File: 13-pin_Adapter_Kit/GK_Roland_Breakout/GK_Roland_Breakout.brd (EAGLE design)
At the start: 40 x 29.6 mm, 39 parts, among them T2 2N4401, U1 RC4558, U2 MIC5205-5V

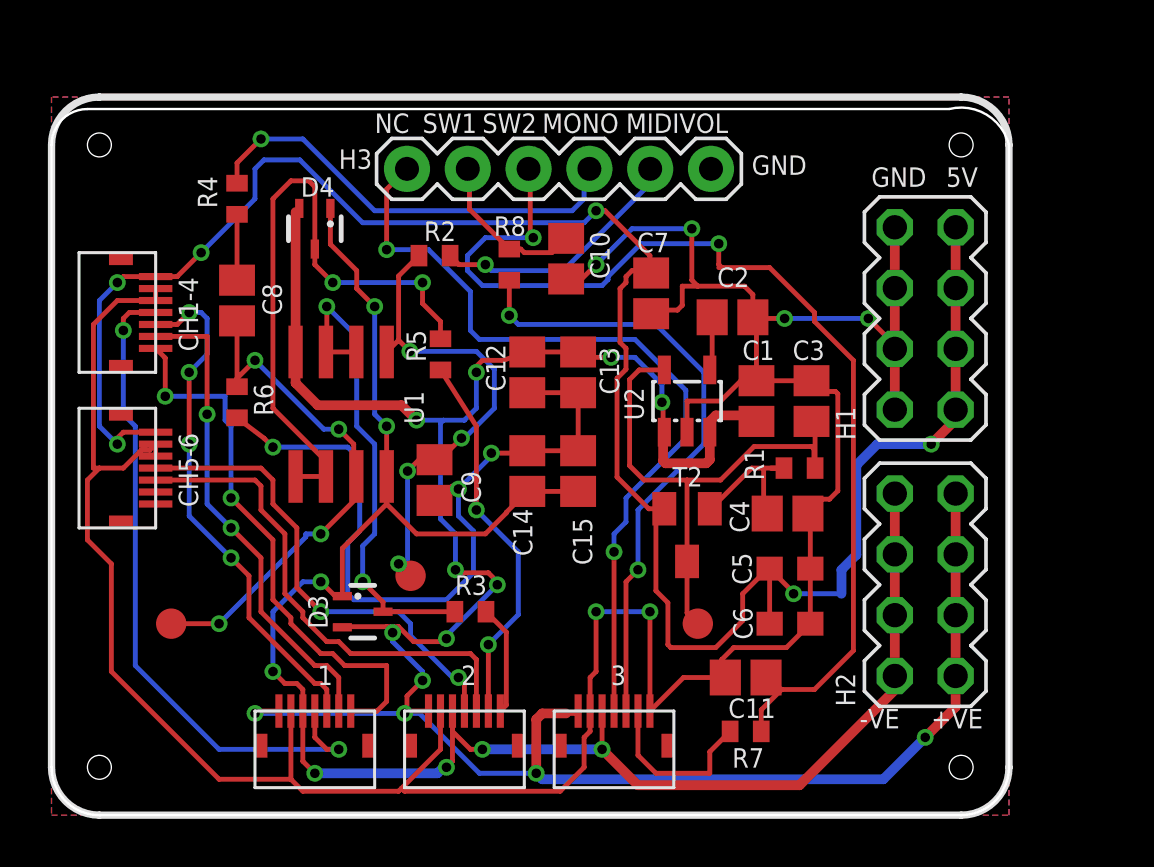
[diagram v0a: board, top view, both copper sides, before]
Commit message: Updated BOM
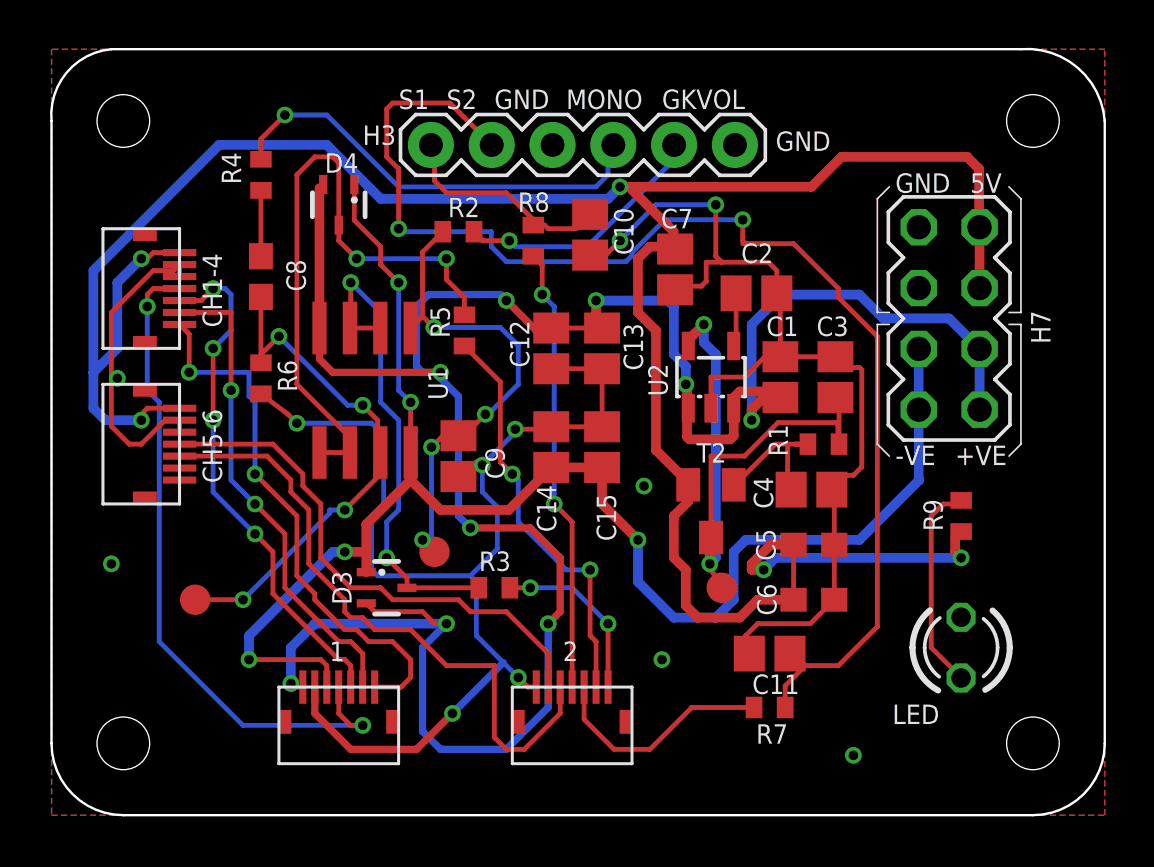
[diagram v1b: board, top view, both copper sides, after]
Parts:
- removed H6, H8: 7P_ZIF_59453-071110EDHLF, CYCFI_Con:7P_ZIF_59453-071110EDHLF
- added LED: (no value), led:LED3MM
- added R9: 4.7k, resistor:R0402
- C10, C11, C9: value 0.01u -> 0.01uF
- C12, C14: value 4.7u -> 4.7uF
- C13, C15: value 0.1u -> 0.1uF
- C5: value 1nf -> 1nF
- C6: value 1uf -> 1uF
- C8: value 0.47u -> 0.47uF; device resistor:C0805 -> resistor:C0603
- H1, H2: value (none) -> 7P_ZIF_59453-071110EDHLF; device con-lstb:MA04-2 -> CYCFI_Con:7P_ZIF_59453-071110EDHLF
- H3: value 6P-2.54-TH -> (none)
- H7: value 7P_ZIF_59453-071110EDHLF -> (none); device CYCFI_Con:7P_ZIF_59453-071110EDHLF -> con-lstb:MA04-2
- R3, R5: value 100 -> 100R
- moved H2 33.3 mm to (3.75, 15.5), turned to 270 degrees
- moved H1 32.8 mm to (3.75, 22.0), turned to 270 degrees
- moved H7 27.1 mm to (37.5, 20.8), turned to 90 degrees
- moved H5 21.8 mm to (21.8, 3.75), turned to 0 degrees
- moved H4 19.6 mm to (12.0, 3.75), turned to 0 degrees
- moved TP1 1.80 mm to (28.0, 9.50)
- moved C1 1.41 mm to (30.4, 18.3)
- moved C10 1.41 mm to (22.5, 24.2)
- moved C11 1.41 mm to (30.0, 6.75)
- moved C12 1.41 mm to (20.9, 19.5)
- moved C13 1.41 mm to (23.0, 19.5)
- moved C14 1.41 mm to (20.9, 15.4)
- moved C15 1.41 mm to (23.0, 15.4)
- moved C2 1.41 mm to (29.4, 21.8)
- moved C3 1.41 mm to (32.8, 18.3)
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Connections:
- removed net N$27: H3.1, H8.P$4
- new net N$2: LED.A, R9.2
- net +VE: now also H4.P$1, H7.1, H7.3; no longer H2.1, H2.3, H2.5, H2.7, H6.P$1, H7.P$1, H8.P$1
- net -VE: now also H4.P$3, H7.2, H7.4; no longer H2.2, H2.4, H2.6, H2.8, H6.P$3, H7.P$3, H8.P$3
- net 5.4V: now also H1.P$1, H2.P$1, H7.5, H7.7, R9.1; no longer H1.1, H1.3, H1.5, H1.7, H4.P$1, H5.P$1
- net GND: now also H1.P$2, H1.P$3, H2.P$2, H2.P$3, H3.3, H5.P$1, H7.6, H7.8, LED.K; no longer H1.2, H1.4, H1.6, H1.8, H4.P$3, H5.P$2, H5.P$3, H6.P$2, H7.P$2, H8.P$2, H8.P$7
- net N$10: now also H2.P$4, H5.P$2; no longer H5.P$4, H7.P$4
- net N$13: now also H5.P$7; no longer H7.P$7
- net N$18: now also H2.P$5, H5.P$3; no longer H5.P$5, H7.P$5
- net N$19: now also H3.1; no longer H3.2
- net N$20: now also H3.2; no longer H3.3
- net N$25: now also H5.P$5; no longer H8.P$6
- net N$26: now also H5.P$4; no longer H8.P$5
- net N$5: now also H1.P$4; no longer H6.P$4
- net N$6: now also H1.P$5; no longer H6.P$5
- net N$7: now also H1.P$6; no longer H6.P$6
- net N$8: now also H1.P$7; no longer H6.P$7
- net N$9: now also H5.P$6; no longer H7.P$6
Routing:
- net GND: track 159.7 -> 104.3 mm, vias 9 -> 12
- net N$27: track 34.3 -> 0.00 mm, vias 2 -> 0
- net 5.4V: track 86.4 -> 104.5 mm, vias 6 -> 5
- net -VE: track 78.4 -> 65.8 mm, vias 8 -> 5
- net N$2: track 0.00 -> 8.81 mm
- net N$20: track 45.4 -> 53.8 mm
- net N$26: track 26.1 -> 18.7 mm
- net N$18: track 20.9 -> 26.4 mm
- net NC1: track 22.8 -> 26.0 mm, vias 0 -> 2
- net N$13: track 4.61 -> 7.37 mm, vias 0 -> 2
- net N$19: track 6.75 -> 9.27 mm
- net N$25: track 7.26 -> 9.69 mm
- net N$10: track 20.1 -> 22.0 mm, vias 2 -> 0
- net N$9: track 15.9 -> 17.1 mm
- net +VE: track 102.8 -> 102.0 mm, vias 13 -> 9
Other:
- board size 40 x 29.6 mm -> 44 x 32 mm
- board text added: "GKVOL"
- board text added: "S1"
- board text added: "S2"
- board text removed: "3"
- board text removed: "C1"
- board text removed: "C10"
- board text removed: "C11"
- board text removed: "C12"
- board text removed: "C13"
- board text removed: "C14"
- board text removed: "C15"
- board text removed: "C2"
- board text removed: "C3"
- board text removed: "C4"
- board text removed: "C5"
- board text removed: "C6"
- board text removed: "C7"
- board text removed: "C8"
- board text removed: "C9"
- board text removed: "H1"
- board text removed: "H2"
- board text removed: "H3"
- board text removed: "MIDIVOL"
- board text removed: "NC"
- board text removed: "R1"
- board text removed: "R2"
- board text removed: "R3"
- board text removed: "R4"
- board text removed: "R5"
- board text removed: "R6"
- board text removed: "R7"
- board text removed: "R8"
- board text removed: "SW1"
- board text removed: "SW2"
- board text removed: "T2"
- board text removed: "TP1"
- board text removed: "TP2"
- board text removed: "TP3"
- board text removed: "U1"
- board text removed: "U2"
- board text removed: "U3"
- board text removed: "U4"
